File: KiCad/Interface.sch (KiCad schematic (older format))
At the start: 22 parts, among them J301 IR LED, J302 Button, SW301 Reset, SW302 Push 1, SW303 Push 2, U301 ULN2003

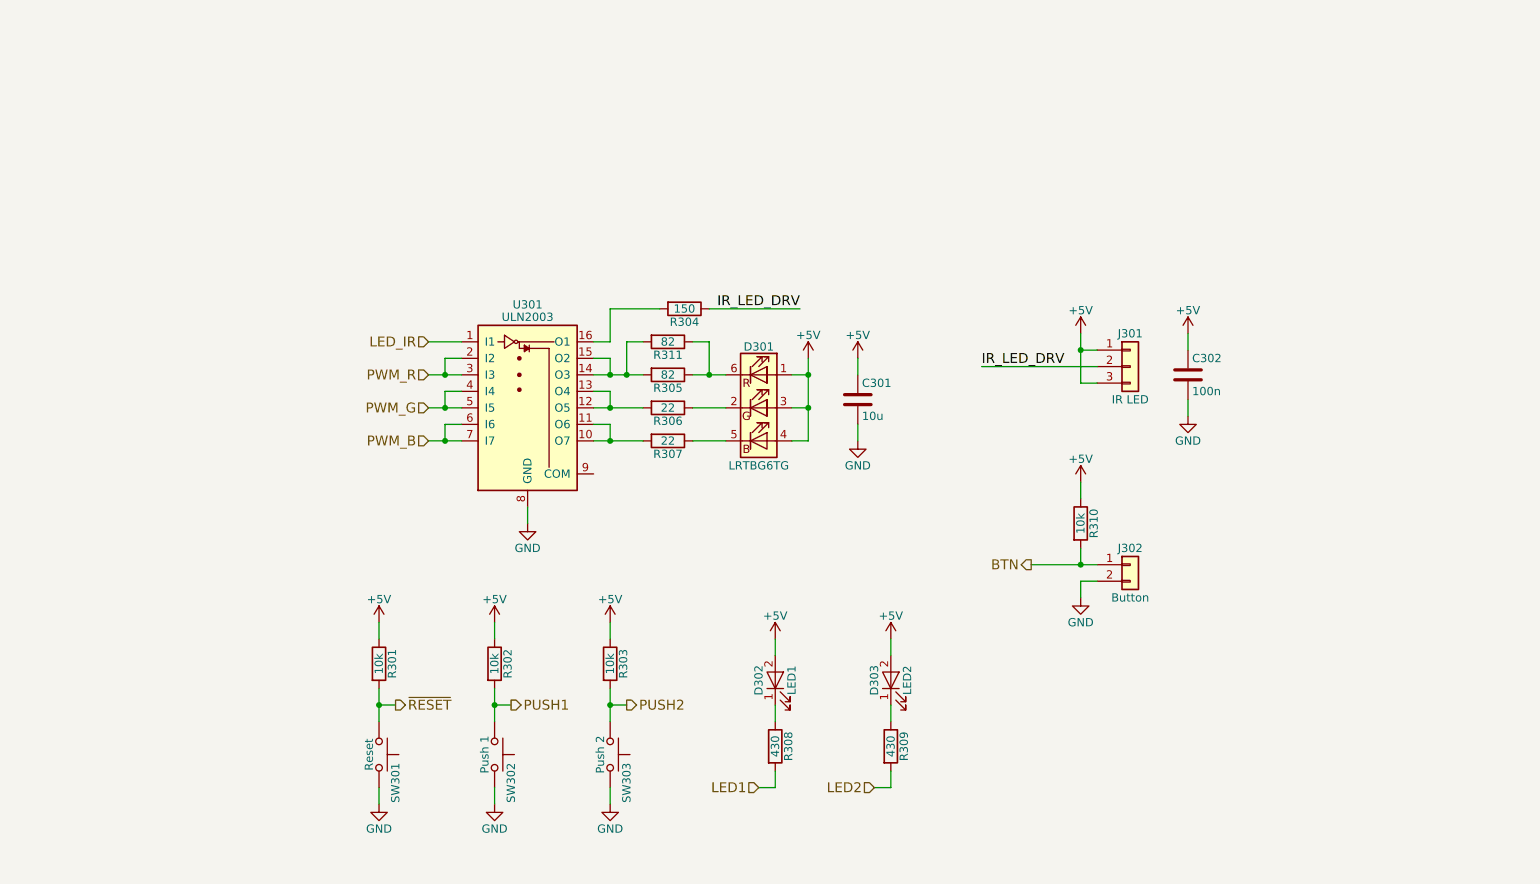
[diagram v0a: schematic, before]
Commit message: Schematic Version 4 Some Software Changes
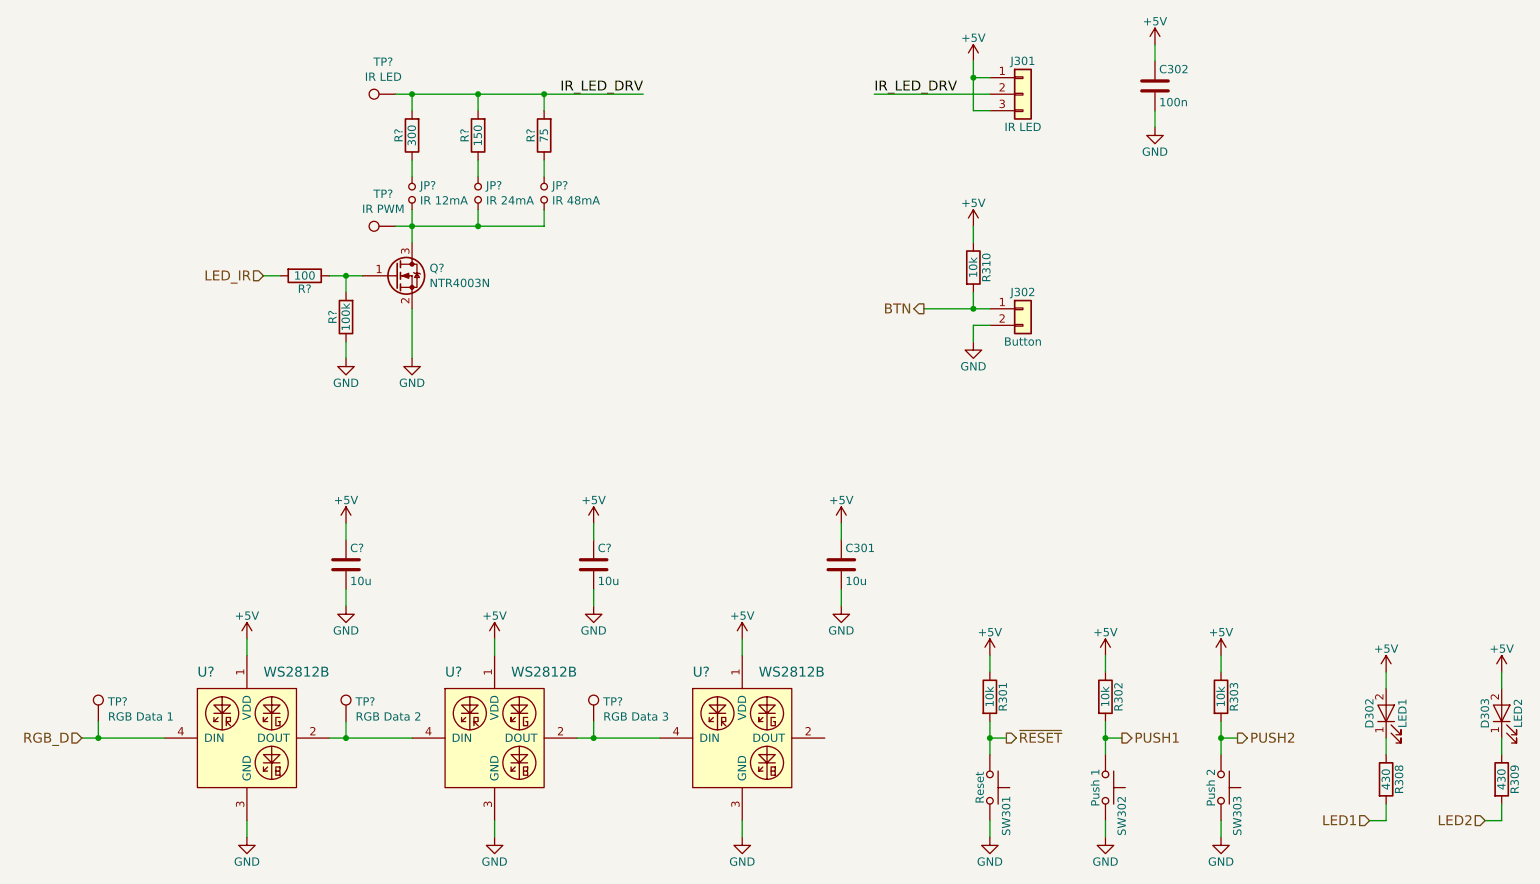
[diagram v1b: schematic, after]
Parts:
- removed D301: LRTBG6TG, ledbox-newfootprints:LED-6-BIG, symbol LRTBG6TG
- removed R304: 150, Resistors_SMD:R_0805, symbol R
- removed R305, R311: 82, Resistors_SMD:R_0805, symbol R
- removed R306, R307: 22, Resistors_SMD:R_0805, symbol R
- removed U301: ULN2003, Housings_SOIC:SOIC-16_3.9x9.9mm_Pitch1.27mm, symbol ULN2003
- added C? (x2): 10u, Capacitors_SMD:C_0805, symbol C
- added JP?: IR 24mA, SMD_Jumper:Jumper_SMD_02, symbol Jumper_NO_Small
- added JP?: IR 48mA, SMD_Jumper:Jumper_SMD_02, symbol Jumper_NO_Small
- added JP?: IR 12mA, SMD_Jumper:Jumper_SMD_02, symbol Jumper_NO_Small
- added Q?: NTR4003N, TO_SOT_Packages_SMD:SOT-23, symbol Q_NMOS_GSD
- added R?: 100, Resistors_SMD:R_0805, symbol R
- added R?: 300, Resistors_SMD:R_0805, symbol R
- added R?: 150, Resistors_SMD:R_0805, symbol R
- added R?: 75, Resistors_SMD:R_0805, symbol R
- added R?: 100k, Resistors_SMD:R_0805, symbol R
- added TP?: IR PWM, symbol Test_Point
- added TP?: RGB Data 1, symbol Test_Point
- added TP?: RGB Data 2, symbol Test_Point
- added TP?: RGB Data 3, symbol Test_Point
- added TP?: IR LED, symbol Test_Point
- added U? (x3): WS2812B, LEDs:LED_WS2812B-PLCC4, symbol WS2812B
- D302, D303: footprint LEDs:LED_0805 -> LEDs:LED_D3.0mm
- SW301, SW302, SW303: Assembly (none) -> DNP
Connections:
- net +5V: now also C?.1, C?.1, U?.1 (VDD), U?.1 (VDD), U?.1 (VDD)
- net GND: now also C?.2, C?.2, Q?.2 (S), R?.1, U?.3 (GND), U?.3 (GND), U?.3 (GND)
- net IR_LED_DRV: now also R?.2, R?.2, R?.2, TP?.1
- net LED_IR: now also R?.2
- new net: Q?.1 (G), R?.1, R?.2
- new net: JP?.2, JP?.2, JP?.2, Q?.3 (D), TP?.1
- new net: JP?.1, R?.1 (x3)
- new net: TP?.1, U?.2 (DOUT), U?.4 (DIN) (x2)
- new net RGB_D: TP?.1, U?.4 (DIN)
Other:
- moved on the sheet: C301, C302, D302, D303, J301, J302, R301, R302, R303, R308, R309, R310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
